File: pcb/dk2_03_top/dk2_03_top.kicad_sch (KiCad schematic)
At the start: 17 parts, among them J1 Conn_01x18_Pin, J2 Euro_Out_1, J2 Euro_Out_2, J2 Sync_In, J2 Sync_Out, J2 Trigger_Out_1, J2 Trigger_Out_2, J2 Trigger_Out_3, J2 Trigger_Out_4, J6 Micro_SD_Card, J7 Conn_01x18_Pin, SW2 SW_Push

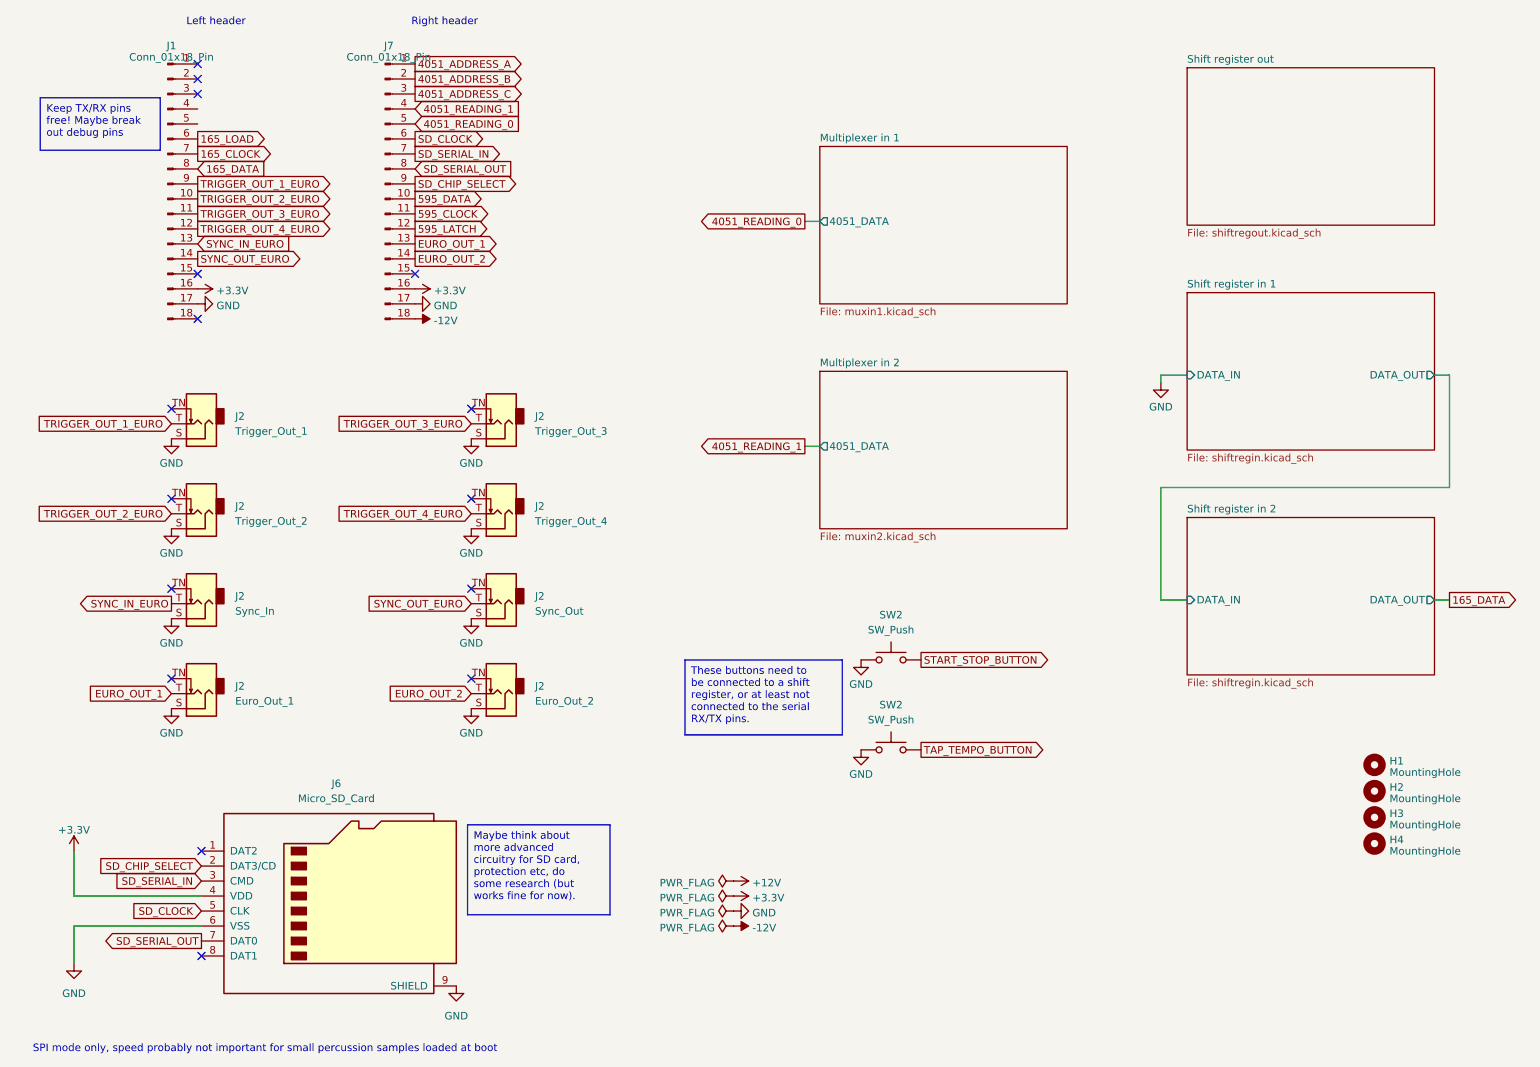
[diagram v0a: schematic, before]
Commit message: pcb progress
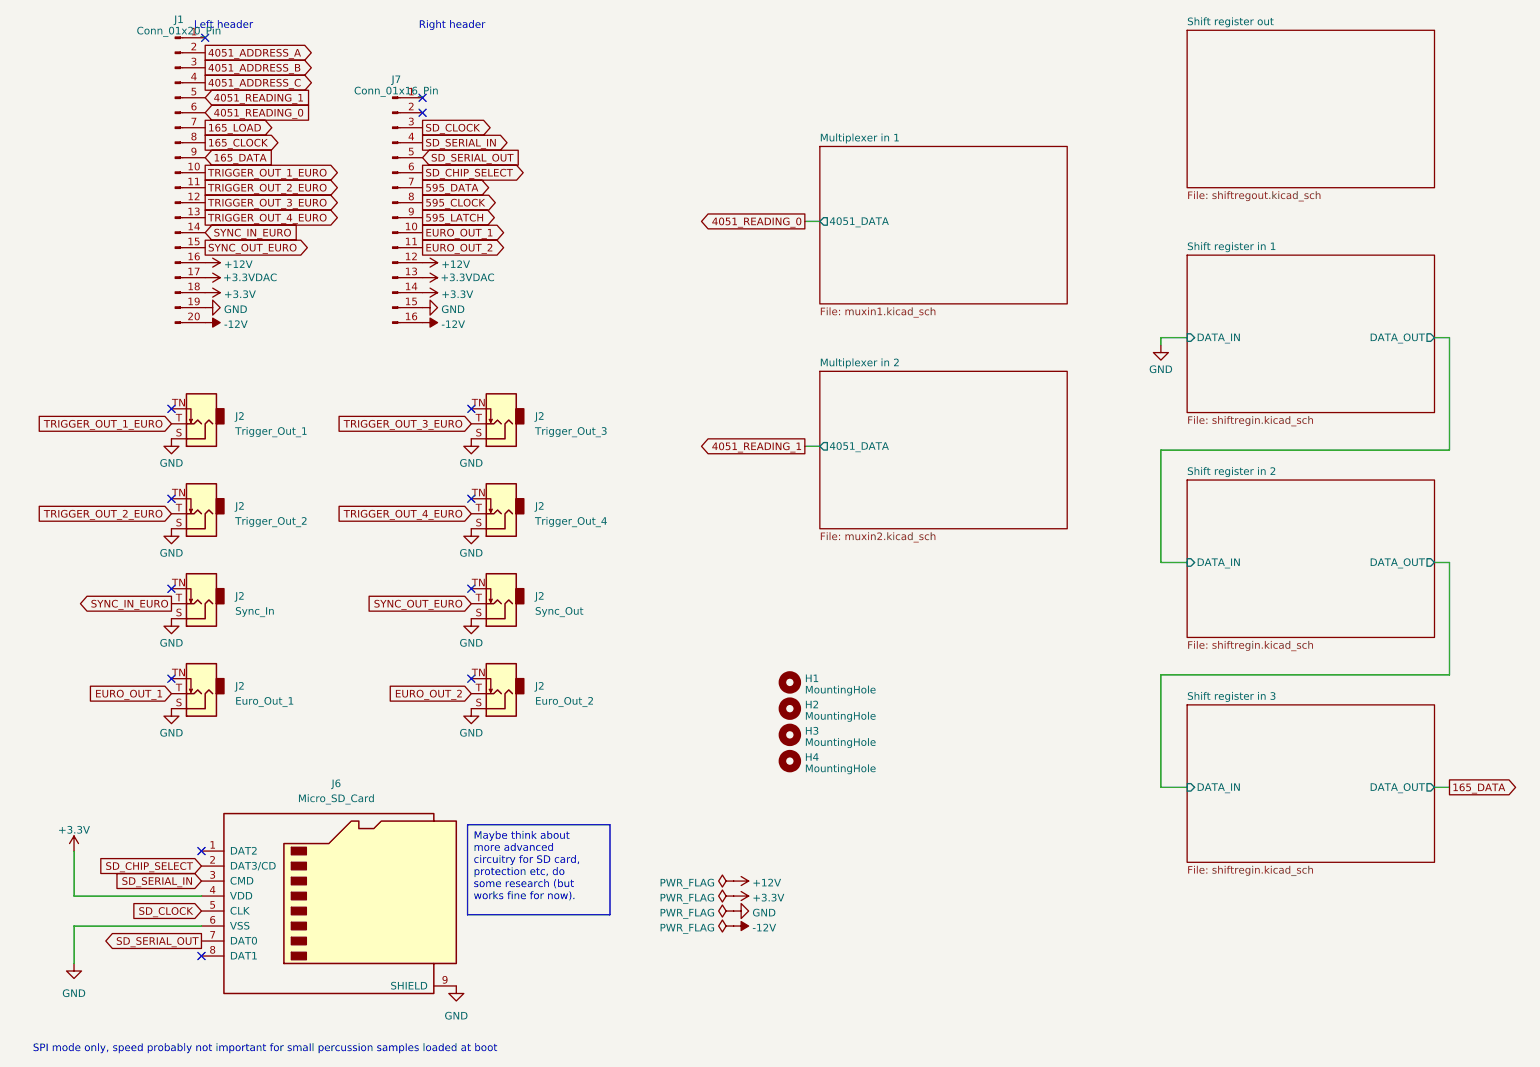
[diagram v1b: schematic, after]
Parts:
- removed J1, J7: Conn_01x18_Pin, Connector_PinHeader_2.54mm:PinHeader_1x18_P2.54mm_Vertical, symbol Connector:Conn_01x18_Pin
- removed SW2 (x2): SW_Push, Button_Switch_THT:SW_PUSH-12mm, symbol Switch:SW_Push
- added J1: Conn_01x20_Pin, symbol Connector:Conn_01x20_Pin
- added J7: Conn_01x16_Pin, symbol Connector:Conn_01x16_Pin
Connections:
- net +12V: now also J1.16 (Pin_16), J7.12 (Pin_12)
- net +3.3V: now also J1.18 (Pin_18), J7.14 (Pin_14)
- net -12V: now also J1.20 (Pin_20), J7.16 (Pin_16)
- net 165_CLOCK: now also J1.8 (Pin_8)
- net 165_DATA: now also J1.9 (Pin_9)
- net 165_LOAD: now also J1.7 (Pin_7)
- net 4051_ADDRESS_A: now also J1.2 (Pin_2)
- net 4051_ADDRESS_B: now also J1.3 (Pin_3)
- net 4051_ADDRESS_C: now also J1.4 (Pin_4)
- net 4051_READING_0: now also J1.6 (Pin_6)
- net 4051_READING_1: now also J1.5 (Pin_5)
- net 595_CLOCK: now also J7.8 (Pin_8)
- net 595_DATA: now also J7.7 (Pin_7)
- net 595_LATCH: now also J7.9 (Pin_9)
- net EURO_OUT_1: now also J7.10 (Pin_10)
- net EURO_OUT_2: now also J7.11 (Pin_11)
- net GND: now also J1.19 (Pin_19), J7.15 (Pin_15)
- net SD_CHIP_SELECT: now also J7.6 (Pin_6)
- net SD_CLOCK: now also J7.3 (Pin_3)
- net SD_SERIAL_IN: now also J7.4 (Pin_4)
- net SD_SERIAL_OUT: now also J7.5 (Pin_5)
- net SYNC_IN_EURO: now also J1.14 (Pin_14)
- net SYNC_OUT_EURO: now also J1.15 (Pin_15)
- net TRIGGER_OUT_1_EURO: now also J1.10 (Pin_10)
- net TRIGGER_OUT_2_EURO: now also J1.11 (Pin_11)
- net TRIGGER_OUT_3_EURO: now also J1.12 (Pin_12)
- net TRIGGER_OUT_4_EURO: now also J1.13 (Pin_13)
- new net +3.3VDAC: J1.17 (Pin_17), J7.13 (Pin_13)
- no-connect marks 16 -> 13
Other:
- added sheet Shift register in 3 (shiftregin.kicad_sch)
- moved on the sheet: H1, H2, H3, H4
